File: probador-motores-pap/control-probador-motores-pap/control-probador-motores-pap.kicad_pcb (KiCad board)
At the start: 2 copper layers, 50 x 35 mm, 11 parts, among them J1 Screw_Terminal_01x06, P1 SW_Push, U1 NE555

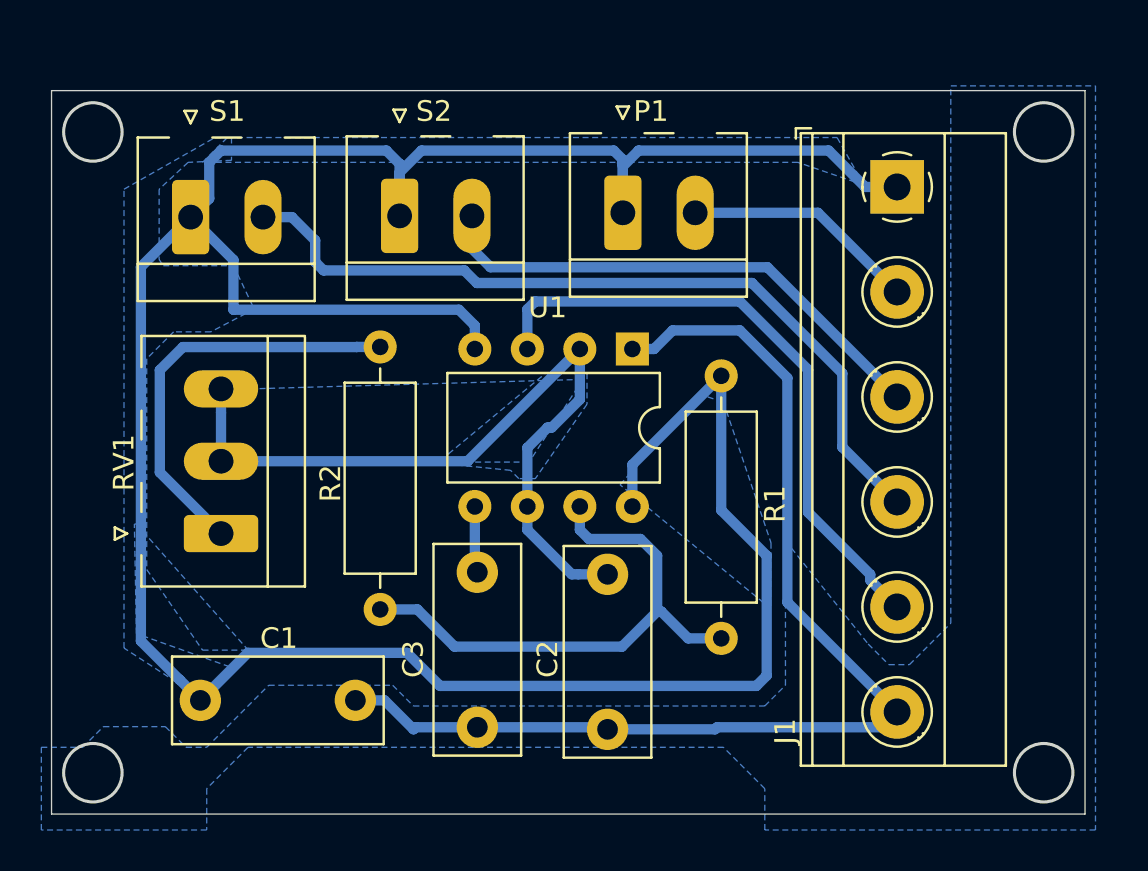
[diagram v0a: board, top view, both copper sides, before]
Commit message: Add files via upload
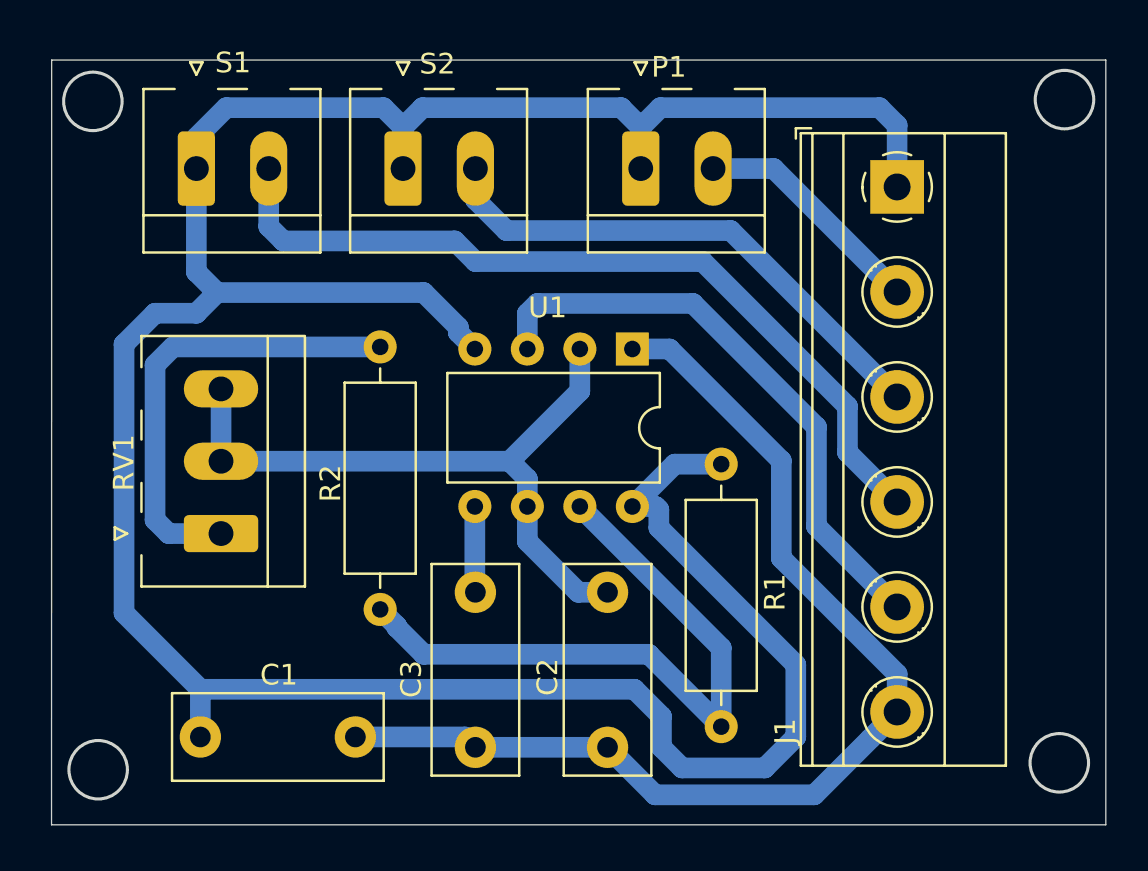
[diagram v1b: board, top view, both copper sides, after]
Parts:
- moved R1 4.27 mm to (133.9, 87.3)
- moved S1 2.37 mm to (108.5, 70.5)
- moved P1 2.31 mm to (130.0, 70.5)
- moved S2 2.30 mm to (118.5, 70.5)
- moved C1 1.77 mm to (108.7, 100.5)
- moved C3 0.97 mm to (122.0, 93.5)
- moved C2 0.87 mm to (128.4, 93.5)
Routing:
- net Net-(R1-Pad2): track 26.6 -> 32.4 mm
- net Net-(C2-Pad1): track 37.8 -> 33.4 mm
- net Net-(R2-Pad2): track 20.3 -> 22.2 mm
- net /Reloj: track 30.3 -> 28.7 mm
- net +5V: track 144.7 -> 143.3 mm
- net /Medio_Full_Paso: track 39.1 -> 40.0 mm
- net Net-(C3-Pad1): track 3.23 -> 4.16 mm
- net /Direccion: track 25.1 -> 25.9 mm
- removed copper zone on B.Cu, net +5V
- removed copper zone on B.Cu, net GND
- removed copper zone on B.Cu, net Net-(C2-Pad1)
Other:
- board size 50 x 35 mm -> 51 x 37 mm
- net class CNC added: clearance 0.5, trace_width 1, via_dia 0.8, via_drill 0.4
- net class Default: clearance 0.2 -> 0.3
- rule solder_mask_min_width: 0.25 -> 0.5
- rule trace_clearance: 0.2 -> 0.3
